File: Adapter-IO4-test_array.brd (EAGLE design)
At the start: 128.3 x 106.7 mm, 89 parts

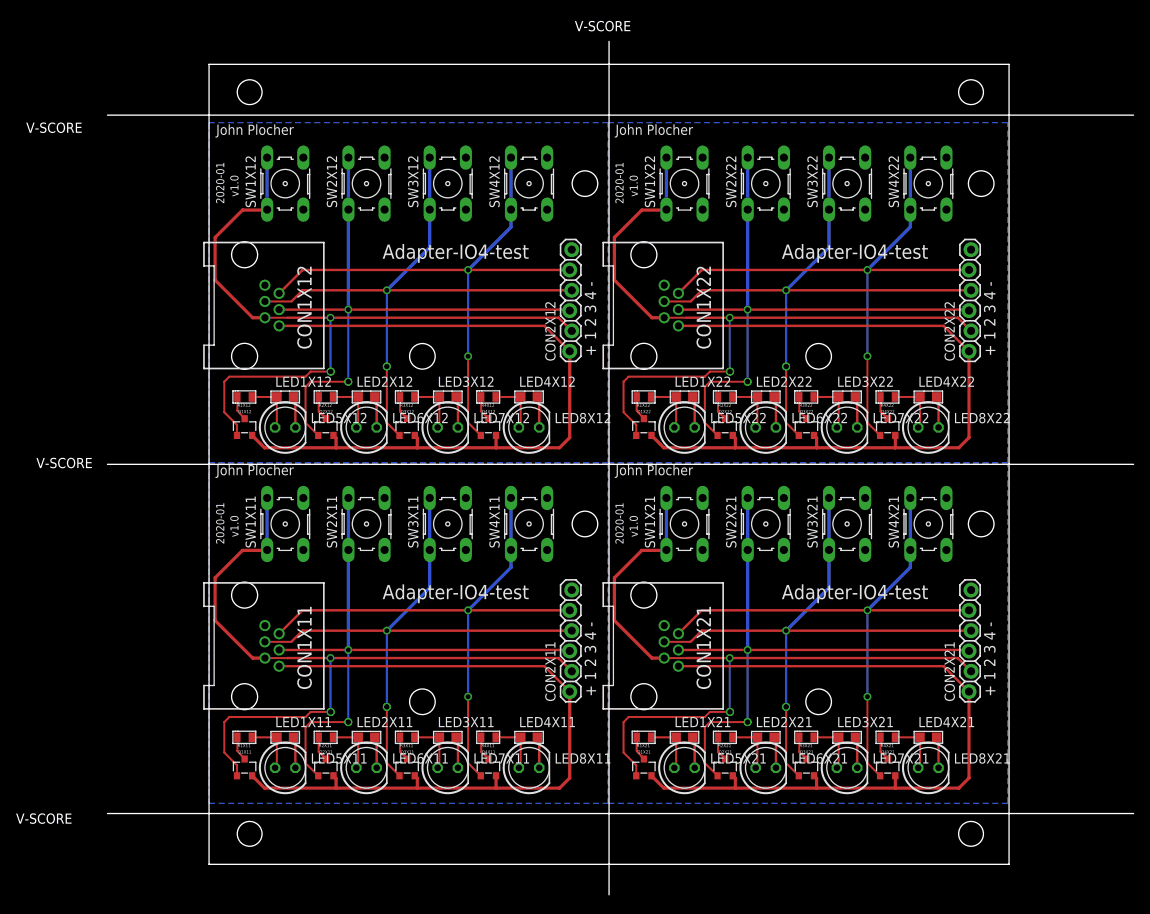
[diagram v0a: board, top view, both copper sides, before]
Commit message: simplified design
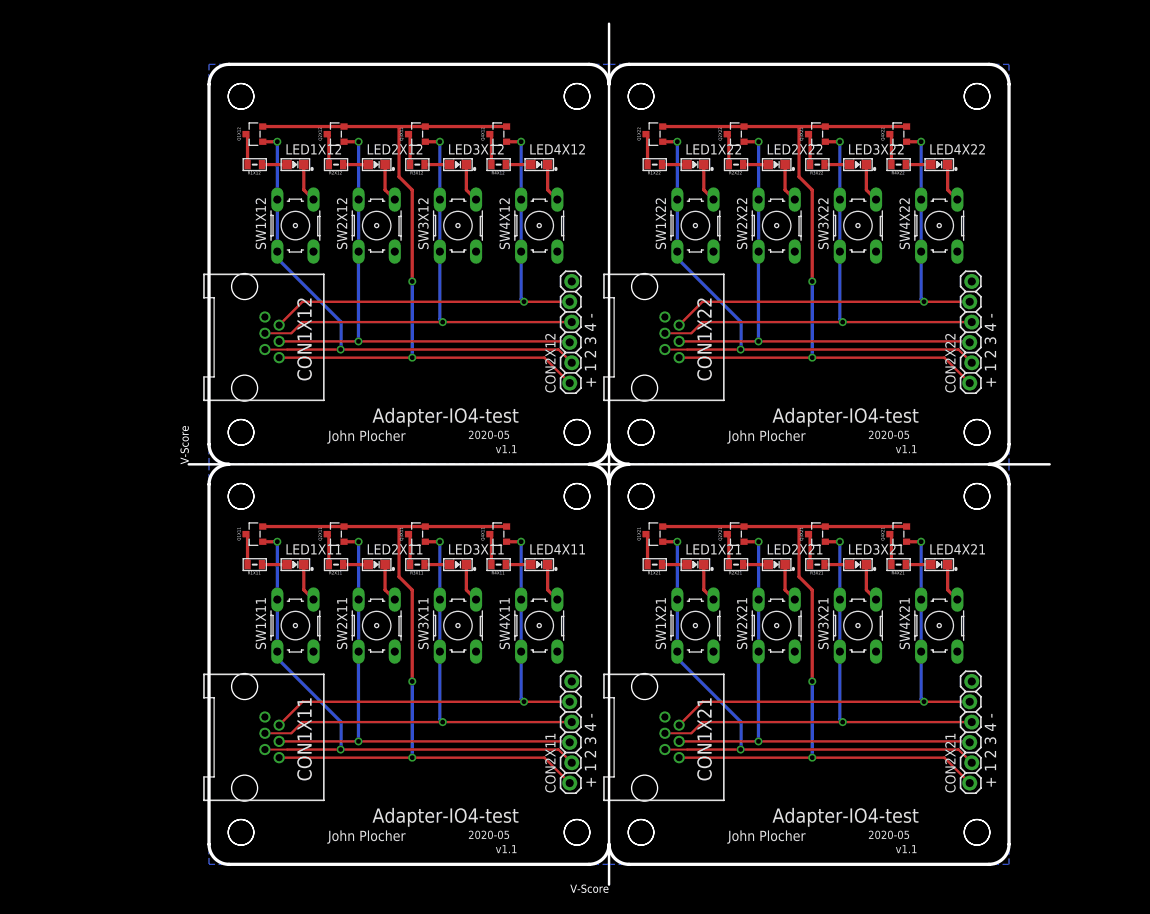
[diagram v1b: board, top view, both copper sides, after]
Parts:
- removed LED5X11, LED5X12, LED5X21, LED5X22, LED6X11, LED6X12, LED6X21, LED6X22, LED7X11, LED7X12, LED7X21, LED7X22, LED8X11, LED8X12, LED8X21, LED8X22: (no value), SPCoast:LED5MM
- removed SW4X1: (no value), SPCoast:BOARD-10X10-2X2-PANEL
- moved Q1X22 36.7 mm to (55.7, 91.3), turned to 90 degrees
- moved Q2X22 36.7 mm to (65.9, 91.3), turned to 90 degrees
- moved Q3X22 36.7 mm to (76.0, 91.3), turned to 90 degrees
- moved Q4X22 36.7 mm to (86.2, 91.3), turned to 90 degrees
- moved Q1X12 36.7 mm to (5.71, 91.3), turned to 90 degrees
- moved Q2X12 36.7 mm to (15.9, 91.3), turned to 90 degrees
- moved Q3X12 36.7 mm to (26.0, 91.3), turned to 90 degrees
- moved Q4X12 36.7 mm to (36.2, 91.3), turned to 90 degrees
- moved Q1X21 29.2 mm to (55.7, 41.3), turned to 90 degrees
- moved Q2X21 29.2 mm to (65.9, 41.3), turned to 90 degrees
- moved Q3X21 29.2 mm to (76.0, 41.3), turned to 90 degrees
- moved Q4X21 29.2 mm to (86.2, 41.3), turned to 90 degrees
- moved Q1X11 29.2 mm to (5.71, 41.3), turned to 90 degrees
- moved Q2X11 29.2 mm to (15.9, 41.3), turned to 90 degrees
- moved Q3X11 29.2 mm to (26.0, 41.3), turned to 90 degrees
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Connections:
- net GNDX11: no longer LED5X11.K, LED6X11.K, LED7X11.K, LED8X11.K
- net GNDX12: no longer LED5X12.K, LED6X12.K, LED7X12.K, LED8X12.K
- net GNDX21: no longer LED5X21.K, LED6X21.K, LED7X21.K, LED8X21.K
- net GNDX22: no longer LED5X22.K, LED6X22.K, LED7X22.K, LED8X22.K
- net N$16X11: no longer LED8X11.A
- net N$16X12: no longer LED8X12.A
- net N$16X21: no longer LED8X21.A
- net N$16X22: no longer LED8X22.A
- net N$2X11: no longer LED5X11.A
- net N$2X12: no longer LED5X12.A
- net N$2X21: no longer LED5X21.A
- net N$2X22: no longer LED5X22.A
- net N$4X11: no longer LED6X11.A
- net N$4X12: no longer LED6X12.A
- net N$4X21: no longer LED6X21.A
- net N$4X22: no longer LED6X22.A
- net N$6X11: no longer LED7X11.A
- net N$6X12: no longer LED7X12.A
- net N$6X21: no longer LED7X21.A
- net N$6X22: no longer LED7X22.A
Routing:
- net N$7X22: track 95.0 -> 70.2 mm
- net N$7X21: track 95.0 -> 70.2 mm
- net N$7X12: track 95.0 -> 70.2 mm
- net N$7X11: track 95.0 -> 70.2 mm
- net N$10X11: track 75.1 -> 59.5 mm
- net N$10X12: track 75.1 -> 59.5 mm
- net N$10X22: track 75.1 -> 59.5 mm
- net N$10X21: track 75.1 -> 59.5 mm
- net N$8X21: track 76.7 -> 63.1 mm, vias 3 -> 2
- net N$8X12: track 76.7 -> 63.1 mm, vias 3 -> 2
- net N$8X22: track 76.7 -> 63.1 mm, vias 3 -> 2
- net N$8X11: track 76.7 -> 63.1 mm, vias 3 -> 2
- net N$9X21: track 76.5 -> 63.4 mm, vias 3 -> 2
- net N$9X22: track 76.5 -> 63.4 mm, vias 3 -> 2
- net N$9X11: track 76.5 -> 63.4 mm, vias 3 -> 2
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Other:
- board size 128.3 x 106.7 mm -> 107.6 x 107.6 mm
- board text added: "2020-05"
- board text added: "V-Score"
- board text added: "v1.1"
- board text removed: "2020-01"
- board text removed: "v1.0"
